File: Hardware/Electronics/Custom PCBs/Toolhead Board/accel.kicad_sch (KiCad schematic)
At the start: 1 part, among them U10 BMI270

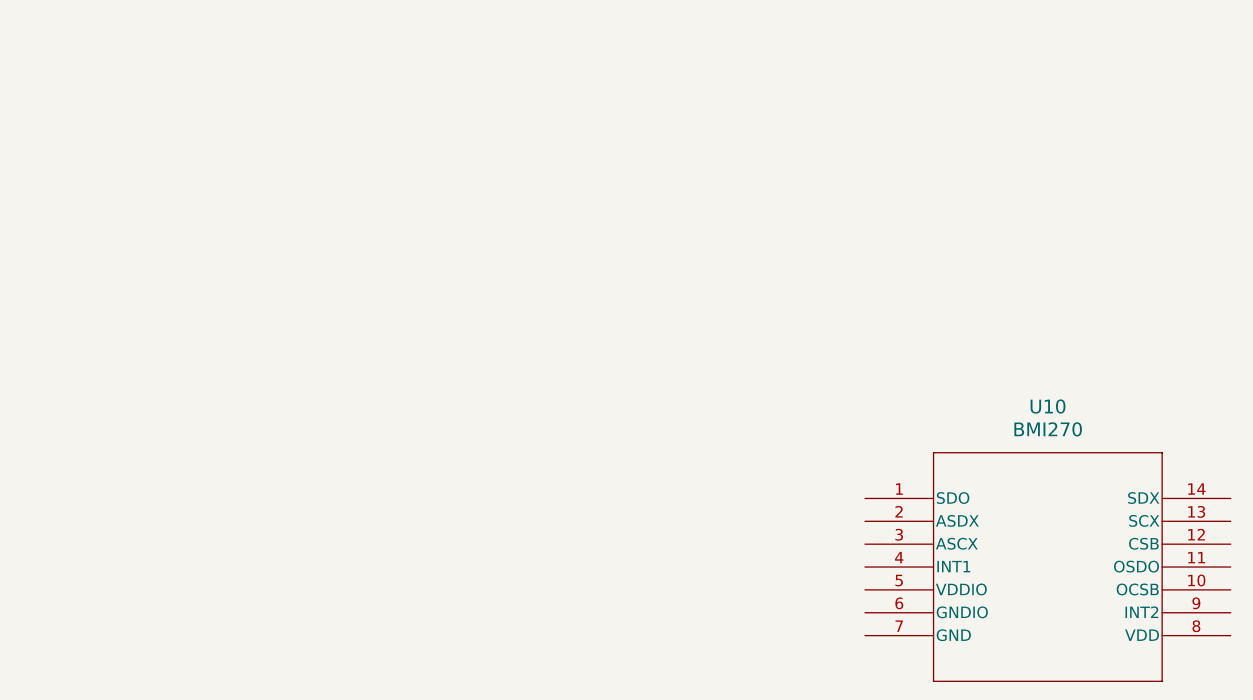
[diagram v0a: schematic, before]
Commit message: Remove locks
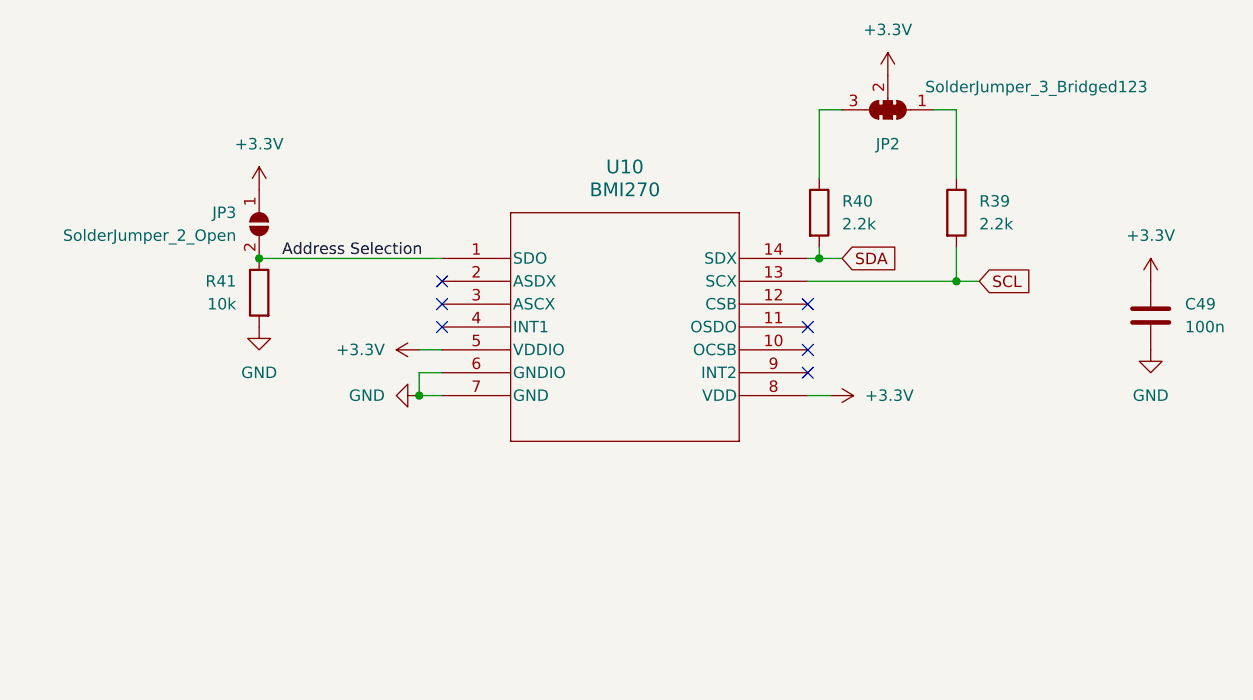
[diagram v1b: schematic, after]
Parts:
- added C49: 100n, symbol Device:C
- added JP2: SolderJumper_3_Bridged123, symbol Jumper:SolderJumper_3_Bridged123
- added JP3: SolderJumper_2_Open, symbol Jumper:SolderJumper_2_Open
- added R39, R40: 2.2k, symbol Device:R
- added R41: 10k, symbol Device:R
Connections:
- net Address Selection: now reaches U10.1 (SDO)
- net Address Selection: now also JP3.2 (B), R41.1
- net SCL: now reaches U10.13 (SCX)
- net SCL: now also R39.2
- net SDA: now reaches U10.14 (SDX)
- net SDA: now also R40.2
- net +3.3V: now reaches U10.5 (VDDIO)
- net +3.3V: now also U10.8 (VDD), C49.1, JP2.2 (C), JP3.1 (A)
- net GND: now reaches U10.6 (GNDIO)
- net GND: now also U10.7 (GND), C49.2, R41.2
- new net: JP2.1 (A), R39.1
- new net: JP2.3 (B), R40.1
- no-connect marks 0 -> 7
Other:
- moved on the sheet: U10
